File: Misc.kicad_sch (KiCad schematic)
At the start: 18 parts, among them J1 BM04B-SURS-TFLFSN, J2 Conn_02x08_Top_Bottom, J3 Conn_01x04, J4 Conn_01x04, J5 Conn_01x05, J501 Conn_01x04, U2 SN65HVD232QDRQ1

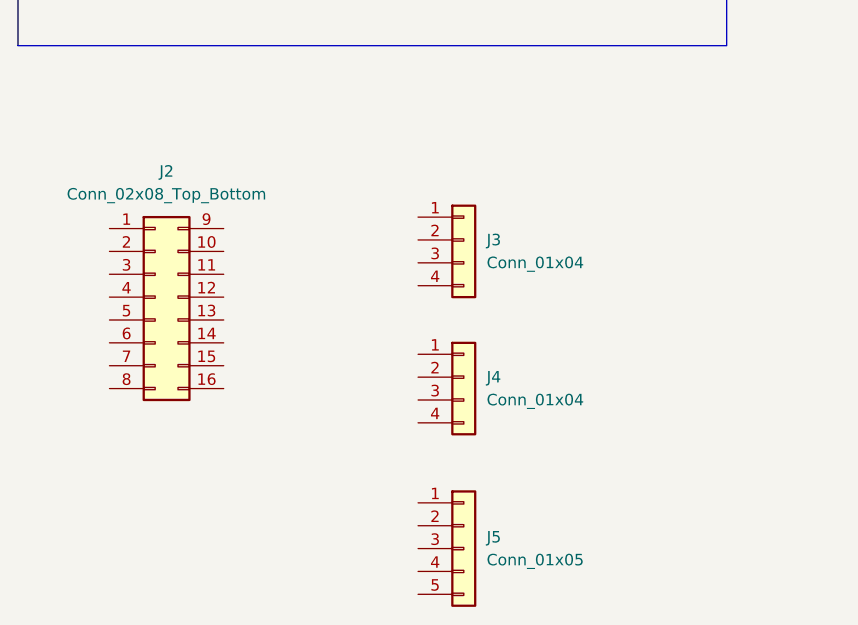
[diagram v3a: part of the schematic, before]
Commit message: this is a message
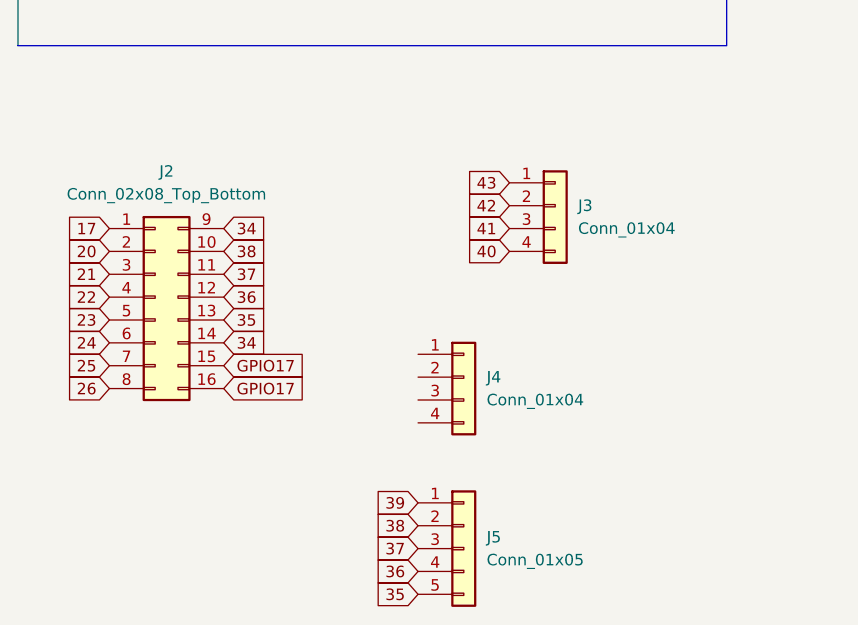
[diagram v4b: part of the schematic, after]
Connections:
- net 17: now reaches J2.1 (Pin_1)
- net 38: now reaches J2.10 (Pin_10)
- net 38: now also J5.2 (Pin_2)
- net 37: now reaches J2.11 (Pin_11)
- net 37: now also J5.3 (Pin_3)
- net 36: now reaches J2.12 (Pin_12)
- net 36: now also J5.4 (Pin_4)
- net 35: now reaches J2.13 (Pin_13)
- net 35: now also J5.5 (Pin_5)
- net 34: now reaches J2.14 (Pin_14)
- net 34: now also J2.9 (Pin_9)
- net GPIO17: now reaches J2.15 (Pin_15)
- net GPIO17: now also J2.16 (Pin_16)
- net 20: now reaches J2.2 (Pin_2)
- net 21: now reaches J2.3 (Pin_3)
- net 22: now reaches J2.4 (Pin_4)
- net 23: now reaches J2.5 (Pin_5)
- net 24: now reaches J2.6 (Pin_6)
- net 25: now reaches J2.7 (Pin_7)
- net 26: now reaches J2.8 (Pin_8)
- net 39: now reaches J5.1 (Pin_1)
- net 43: now reaches J3.1 (Pin_1)
- net 42: now reaches J3.2 (Pin_2)
- net 41: now reaches J3.3 (Pin_3)
- net 40: now reaches J3.4 (Pin_4)
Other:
- moved on the sheet: J3
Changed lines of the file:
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@@
     (effects (font (size 0.4064 0.4064)) (justify left bottom))
   )
+  (global_label "37" (shape input) (at 52.07 82.55 0) (fields_autoplaced)
+    (effects (font (size 1.27 1.27)) (justify left))
+    (property "Intersheet References" "${INTERSHEET_REFS}" (id 0) (at 56.8132 82.4706 0)
+      (effects (font (size 1.27 1.27)) (justify left) hide)
+    )
+  )
+  (global_label "41" (shape input) (at 83.82 77.47 180) (fields_autoplaced)
+    (effects (font (size 1.27 1.27)) (justify right))
+    (property "Intersheet References" "${INTERSHEET_REFS}" (id 0) (at 79.0768 77.3906 0)
+      (effects (font (size 1.27 1.27)) (justify right) hide)
+    )
+  )
+  (global_label "36" (shape input) (at 52.07 85.09 0) (fields_autoplaced)
+    (effects (font (size 1.27 1.27)) (justify left))
+    (property "Intersheet References" "${INTERSHEET_REFS}" (id 0) (at 56.8132 85.0106 0)
+      (effects (font (size 1.27 1.27)) (justify left) hide)
+    )
+  )
+  (global_label "35" (shape input) (at 52.07 87.63 0) (fields_autoplaced)
+    (effects (font (size 1.27 1.27)) (justify left))
+    (property "Intersheet References" "${INTERSHEET_REFS}" (id 0) (at 56.8132 87.5506 0)
+      (effects (font (size 1.27 1.27)) (justify left) hide)
+    )
+  )
+  (global_label "39" (shape input) (at 73.66 107.95 180) (fields_autoplaced)
+    (effects (font (size 1.27 1.27)) (justify right))
+    (property "Intersheet References" "${INTERSHEET_REFS}" (id 0) (at 68.9168 108.0294 0)
+      (effects (font (size 1.27 1.27)) (justify right) hide)
+    )
+  )
+  (global_label "24" (shape input) (at 39.37 90.17 180) (fields_autoplaced)
+    (effects (font (size 1.27 1.27)) (justify right))
+    (property "Intersheet References" "${INTERSHEET_REFS}" (id 0) (at 34.6268 90.0906 0)
+      (effects (font (size 1.27 1.27)) (justify right) hide)
+    )
+  )
+  (global_label "GPIO17" (shape input) (at 52.07 92.71 0) (fields_autoplaced)
+    (effects (font (size 1.27 1.27)) (justify left))
+    (property "Intersheet References" "${INTERSHEET_REFS}" (id 0) (at 61.2885 92.7894 0)
+      (effects (font (size 1.27 1.27)) (justify left) hide)
+    )
+  )
+  (global_label "25" (shape input) (at 39.37 92.71 180) (fields_autoplaced)
+    (effects (font (size 1.27 1.27)) (justify right))
+    (property "Intersheet References" "${INTERSHEET_REFS}" (id 0) (at 34.6268 92.6306 0)
+      (effects (font (size 1.27 1.27)) (justify right) hide)
+    )
+  )
+  (global_label "34" (shape input) (at 52.07 90.17 0) (fields_autoplaced)
+    (effects (font (size 1.27 1.27)) (justify left))
+    (property "Intersheet References" "${INTERSHEET_REFS}" (id 0) (at 56.8132 90.0906 0)
+      (effects (font (size 1.27 1.27)) (justify left) hide)
+    )
+  )
+  (global_label "43" (shape input) (at 83.82 72.39 180) (fields_autoplaced)
+    (effects (font (size 1.27 1.27)) (justify right))
+    (property "Intersheet References" "${INTERSHEET_REFS}" (id 0) (at 79.0768 72.3106 0)
+      (effects (font (size 1.27 1.27)) (justify right) hide)
+    )
+  )
+  (global_label "17" (shape input) (at 39.37 77.47 180) (fields_autoplaced)
+    (effects (font (size 1.27 1.27)) (justify right))
+    (property "Intersheet References" "${INTERSHEET_REFS}" (id 0) (at 34.6268 77.3906 0)
+      (effects (font (size 1.27 1.27)) (justify right) hide)
+    )
+  )
+  (global_label "26" (shape input) (at 39.37 95.25 180) (fields_autoplaced)
+    (effects (font (size 1.27 1.27)) (justify right))
+    (property "Intersheet References" "${INTERSHEET_REFS}" (id 0) (at 34.6268 95.1706 0)
+      (effects (font (size 1.27 1.27)) (justify right) hide)
+    )
+  )
+  (global_label "22" (shape input) (at 39.37 85.09 180) (fields_autoplaced)
+    (effects (font (size 1.27 1.27)) (justify right))
+    (property "Intersheet References" "${INTERSHEET_REFS}" (id 0) (at 34.6268 85.0106 0)
+      (effects (font (size 1.27 1.27)) (justify right) hide)
+    )
+  )
+  (global_label "23" (shape input) (at 39.37 87.63 180) (fields_autoplaced)
+    (effects (font (size 1.27 1.27)) (justify right))
+    (property "Intersheet References" "${INTERSHEET_REFS}" (id 0) (at 34.6268 87.5506 0)
+      (effects (font (size 1.27 1.27)) (justify right) hide)
+    )
+  )
+  (global_label "21" (shape input) (at 39.37 82.55 180) (fields_autoplaced)
+    (effects (font (size 1.27 1.27)) (justify right))
+    (property "Intersheet References" "${INTERSHEET_REFS}" (id 0) (at 34.6268 82.4706 0)
+      (effects (font (size 1.27 1.27)) (justify right) hide)
+    )
+  )
+  (global_label "38" (shape input) (at 73.66 110.49 180) (fields_autoplaced)
+    (effects (font (size 1.27 1.27)) (justify right))
+    (property "Intersheet References" "${INTERSHEET_REFS}" (id 0) (at 68.9168 110.5694 0)
+      (effects (font (size 1.27 1.27)) (justify right) hide)
+    )
+  )
+  (global_label "40" (shape input) (at 83.82 80.01 180) (fields_autoplaced)
+    (effects (font (size 1.27 1.27)) (justify right))
+    (property "Intersheet References" "${INTERSHEET_REFS}" (id 0) (at 79.0768 79.9306 0)
+      (effects (font (size 1.27 1.27)) (justify right) hide)
+    )
+  )
   (global_label "MCU_CAN1_RX" (shape input) (at 149.86 46.99 180) (fields_autoplaced)
     (effects (font (size 1.27 1.27)) (justify right))
@@
     )
   )
+  (global_label "GPIO17" (shape input) (at 52.07 95.25 0) (fields_autoplaced)
+    (effects (font (size 1.27 1.27)) (justify left))
+    (property "Intersheet References" "${INTERSHEET_REFS}" (id 0) (at 61.2885 95.3294 0)
+      (effects (font (size 1.27 1.27)) (justify left) hide)
+    )
+  )
+  (global_label "34" (shape input) (at 52.07 77.47 0) (fields_autoplaced)
+    (effects (font (size 1.27 1.27)) (justify left))
+    (property "Intersheet References" "${INTERSHEET_REFS}" (id 0) (at 56.8132 77.3906 0)
+      (effects (font (size 1.27 1.27)) (justify left) hide)
+    )
+  )
+  (global_label "42" (shape input) (at 83.82 74.93 180) (fields_autoplaced)
+    (effects (font (size 1.27 1.27)) (justify right))
+    (property "Intersheet References" "${INTERSHEET_REFS}" (id 0) (at 79.0768 74.8506 0)
+      (effects (font (size 1.27 1.27)) (justify right) hide)
+    )
+  )
+  (global_label "36" (shape input) (at 73.66 115.57 180) (fields_autoplaced)
+    (effects (font (size 1.27 1.27)) (justify right))
+    (property "Intersheet References" "${INTERSHEET_REFS}" (id 0) (at 68.9168 115.6494 0)
+      (effects (font (size 1.27 1.27)) (justify right) hide)
+    )
+  )
+  (global_label "37" (shape input) (at 73.66 113.03 180) (fields_autoplaced)
+    (effects (font (size 1.27 1.27)) (justify right))
+    (property "Intersheet References" "${INTERSHEET_REFS}" (id 0) (at 68.9168 113.1094 0)
+      (effects (font (size 1.27 1.27)) (justify right) hide)
+    )
+  )
+  (global_label "35" (shape input) (at 73.66 118.11 180) (fields_autoplaced)
+    (effects (font (size 1.27 1.27)) (justify right))
+    (property "Intersheet References" "${INTERSHEET_REFS}" (id 0) (at 68.9168 118.1894 0)
+      (effects (font (size 1.27 1.27)) (justify right) hide)
+    )
+  )
+  (global_label "20" (shape input) (at 39.37 80.01 180) (fields_autoplaced)
+    (effects (font (size 1.27 1.27)) (justify right))
+    (property "Intersheet References" "${INTERSHEET_REFS}" (id 0) (at 34.6268 79.9306 0)
+      (effects (font (size 1.27 1.27)) (justify right) hide)
+    )
+  )
   (global_label "MCU_CAN1_TX" (shape input) (at 149.86 44.45 180) (fields_autoplaced)
     (effects (font (size 1.27 1.27)) (justify right))
     (property "Intersheet References" "${INTERSHEET_REFS}" (id 0) (at 40.64 -91.44 0)
       (effects (font (size 1.27 1.27)) hide)
+    )
+  )
+  (global_label "38" (shape input) (at 52.07 80.01 0) (fields_autoplaced)
+    (effects (font (size 1.27 1.27)) (justify left))
+    (property "Intersheet References" "${INTERSHEET_REFS}" (id 0) (at 56.8132 79.9306 0)
+      (effects (font (size 1.27 1.27)) (justify left) hide)
     )
   )
@@
     (pin "1")
   )
-  (symbol (lib_id "Connector_Generic:Conn_01x04") (at 78.74 78.74 0) (unit 1)
+  (symbol (lib_id "Connector_Generic:Conn_01x04") (at 88.9 74.93 0) (unit 1)
     (in_bom yes) (on_board yes) (fields_autoplaced)
-    (property "Reference" "J3" (id 0) (at 81.28 78.7399 0)
-      (effects (font (size 1.27 1.27)) (justify left))
-    )
-    (property "Value" "Conn_01x04" (id 1) (at 81.28 81.2799 0)
-      (effects (font (size 1.27 1.27)) (justify left))
-    )
-    (property "Footprint" "Connector_PinSocket_2.54mm:PinSocket_1x04_P2.54mm_Vertical" (id 2) (at 78.74 78.74 0)
-      (effects (font (size 1.27 1.27)) hide)
-    )
-    (property "Datasheet" "~" (id 3) (at 78.74 78.74 0)
-      (effects (font (size 1.27 1.27)) hide)
-    )
+    (property "Reference" "J3" (id 0) (at 91.44 74.9299 0)
+      (effects (font (size 1.27 1.27)) (justify left))
+    )
+    (property "Value" "Conn_01x04" (id 1) (at 91.44 77.4699 0)
+      (effects (font (size 1.27 1.27)) (justify left))
+    )
+    (property "Footprint" "Connector_PinSocket_2.54mm:PinSocket_1x04_P2.54mm_Vertical" (id 2) (at 88.9 74.93 0)
+      (effects (font (size 1.27 1.27)) hide)
+    )
+    (property "Datasheet" "~" (id 3) (at 88.9 74.93 0)
+      (effects (font (size 1.27 1.27)) hide)
+    )
